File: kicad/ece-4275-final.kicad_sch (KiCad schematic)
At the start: 10 parts, among them U1 ESP32-S3

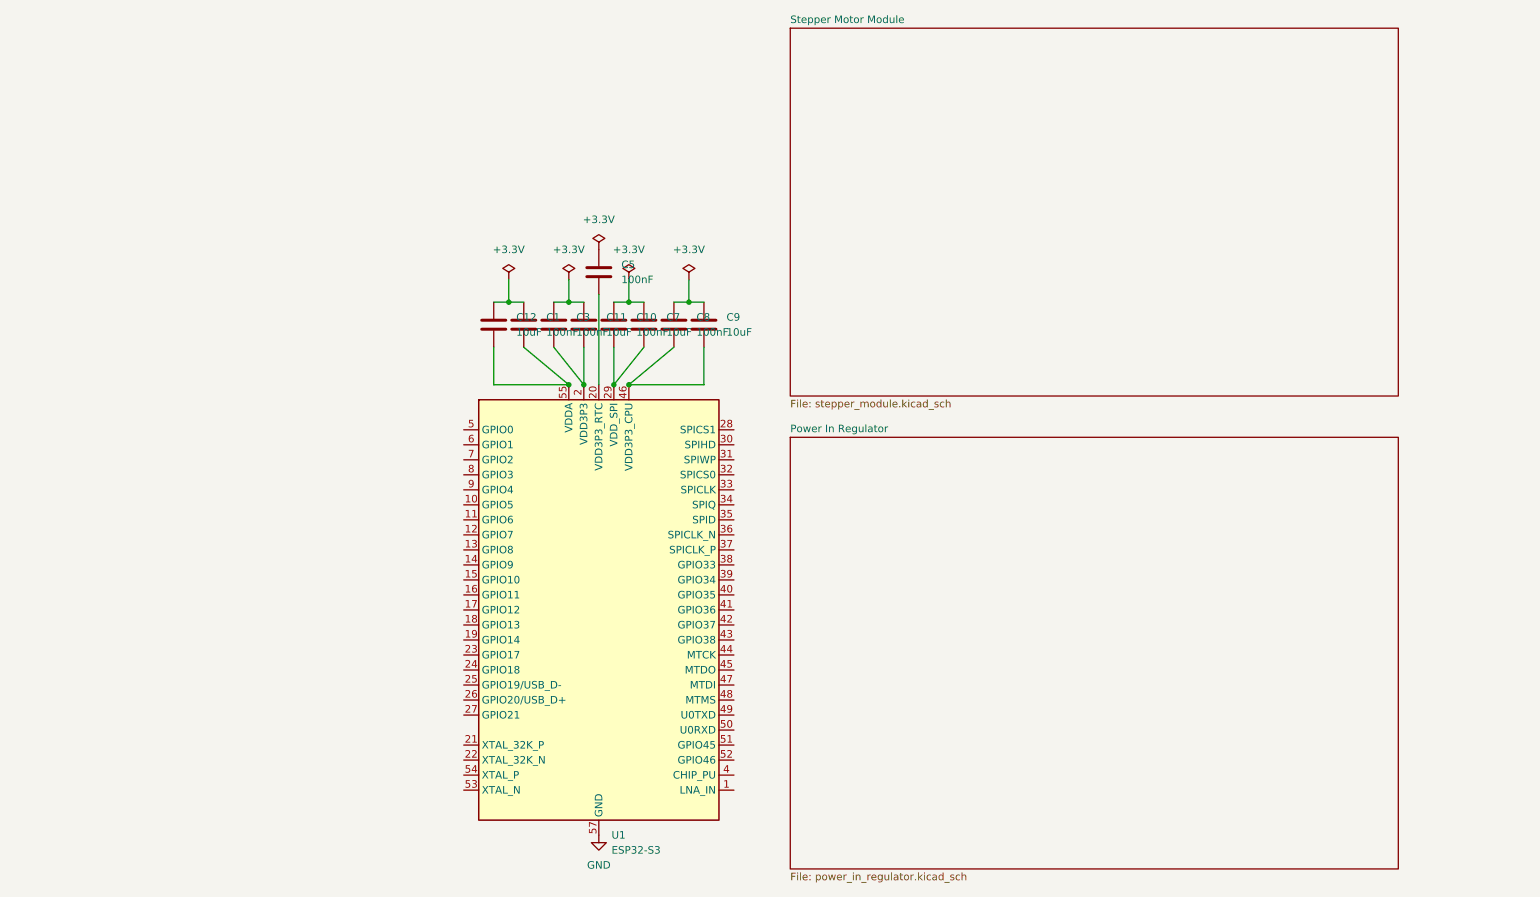
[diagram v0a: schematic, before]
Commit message: finish motor driver module
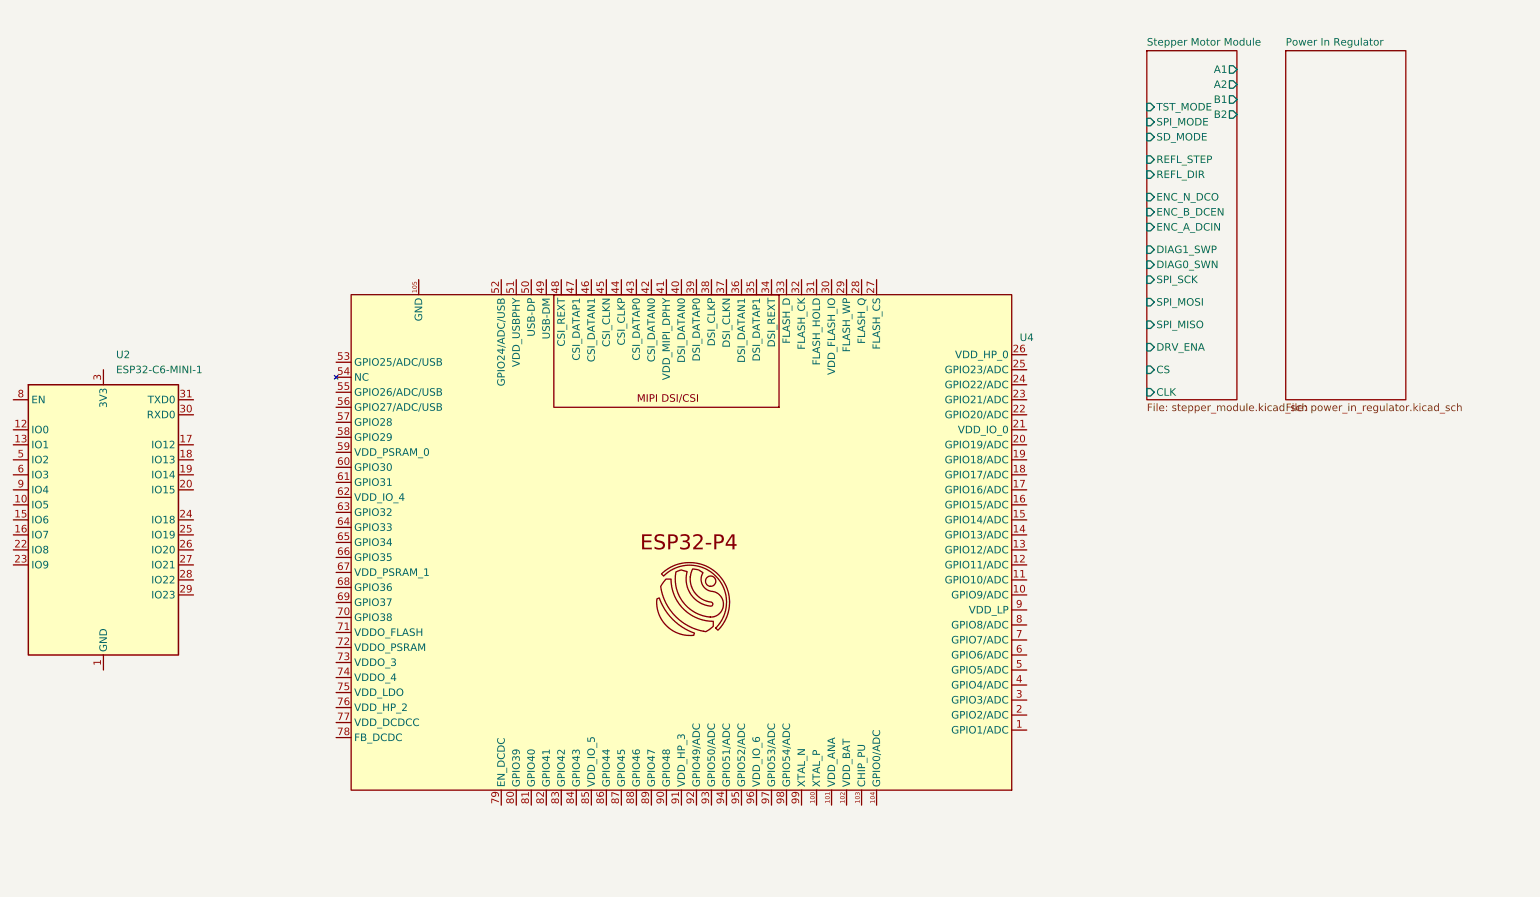
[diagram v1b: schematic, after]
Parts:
- removed C1, C10, C3, C5, C8: 100nF, symbol Device:C
- removed C11, C12, C7, C9: 10uF, symbol Device:C
- removed U1: ESP32-S3, Package_DFN_QFN:QFN-56-1EP_7x7mm_P0.4mm_EP4x4mm, symbol MCU_Espressif:ESP32-S3
- added U2: ESP32-C6-MINI-1, RF_Module:ESP32-C6-MINI-1, symbol RF_Module:ESP32-C6-MINI-1
- added U4: (no value), PCM_Espressif:ESP32-P4, symbol PCM_Espressif:ESP32-P4
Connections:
- new net: U2.1 (GND), U2.11 (GND), U2.14 (GND), U2.2 (GND), U2.36 (GND), U2.37 (GND), U2.38 (GND), U2.39 (GND), U2.40 (GND), U2.41 (GND), U2.42 (GND), U2.43 (GND), U2.44 (GND), U2.45 (GND), U2.46 (GND), U2.47 (GND), U2.48 (GND), U2.49 (GND), U2.50 (GND), U2.51 (GND), U2.52 (GND), U2.53 (GND)
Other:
- sheet Stepper Motor Module ports: added A1, A2, B1, B2, CLK, CS, DIAG0_SWN, DIAG1_SWP, DRV_ENA, ENC_A_DCIN, ENC_B_DCEN, ENC_N_DCO, REFL_DIR, REFL_STEP, SD_MODE, SPI_MISO, SPI_MODE, SPI_MOSI, SPI_SCK, TST_MODE; removed none
